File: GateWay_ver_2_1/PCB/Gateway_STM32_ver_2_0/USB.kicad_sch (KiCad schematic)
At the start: 9 parts, among them J13 USB_A, U17 TPD2EUSB30, U21 TPS2041C

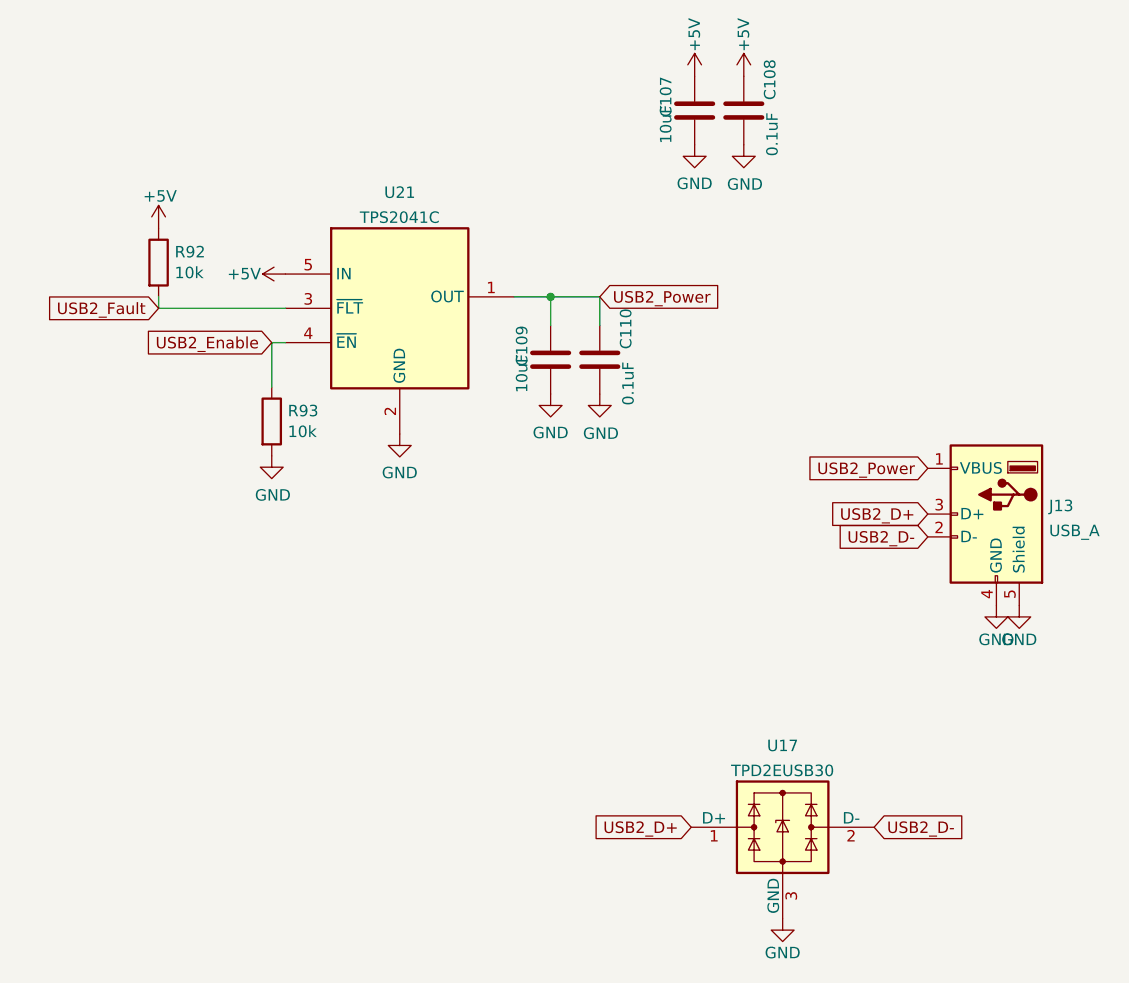
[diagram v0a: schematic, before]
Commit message: 1
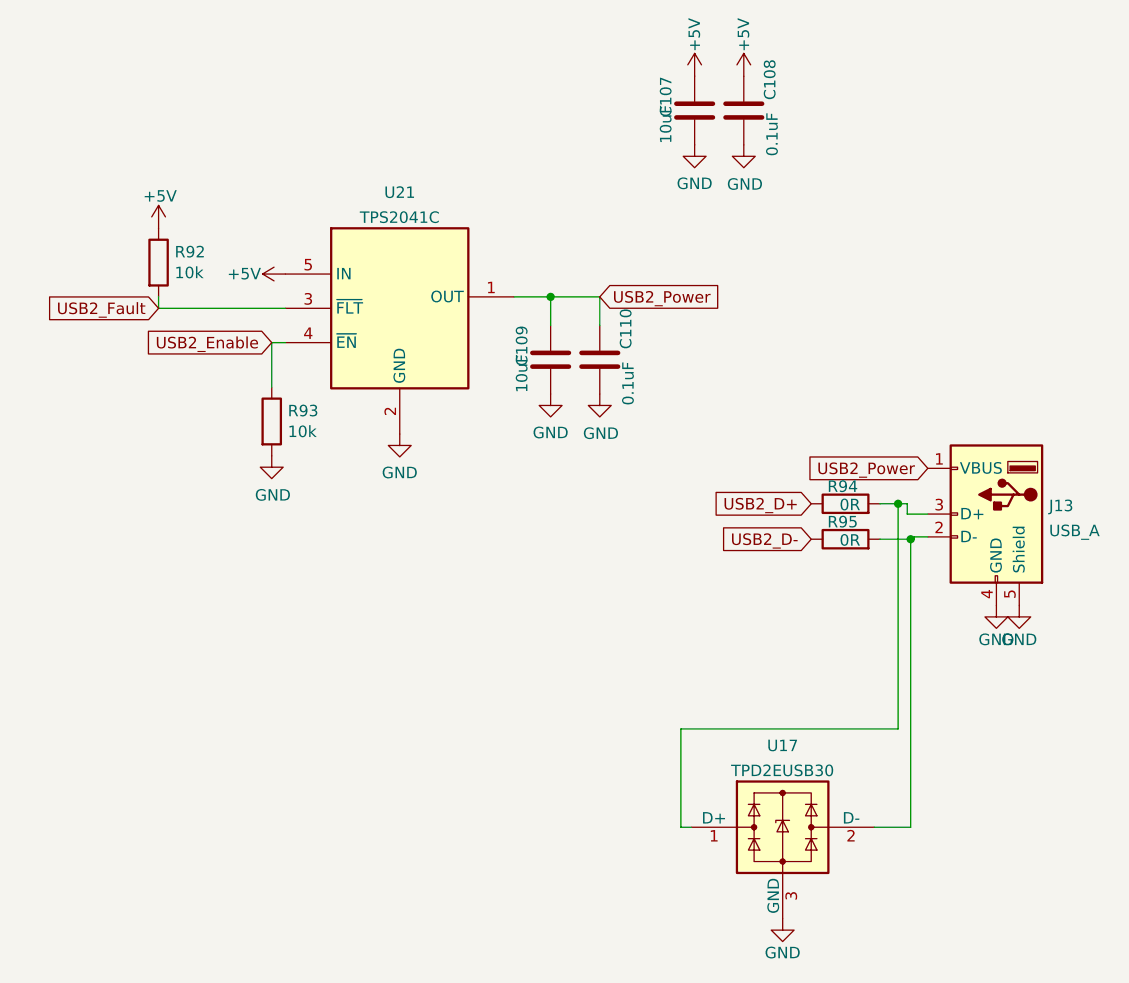
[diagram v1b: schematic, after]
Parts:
- added R94, R95: 0R, Resistor_SMD:R_0603_1608Metric, symbol Device:R
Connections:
- net USB2_D+: now also R94.1; no longer J13.3 (D+), U17.1 (D+)
- net USB2_D-: now also R95.1; no longer J13.2 (D-), U17.2 (D-)
- new net: J13.3 (D+), R94.2, U17.1 (D+)
- new net: J13.2 (D-), R95.2, U17.2 (D-)
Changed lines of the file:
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@@
 (kicad_sch (version 20211123) (generator eeschema)
   (paper "A4")
+  (junction (at 195.58 80.137) (diameter 0) (color 0 0 0 0)
+  )
   (junction (at 156.972 57.15) (diameter 0) (color 0 0 0 0)
   )
+  (junction (at 196.977 84.074) (diameter 0) (color 0 0 0 0)
+  )
+  (wire (pts (xy 195.58 105.156) (xy 195.58 80.137))
+    (stroke (width 0) (type default) (color 0 0 0 0))
+  )
+  (wire (pts (xy 171.45 105.156) (xy 195.58 105.156))
+    (stroke (width 0) (type default) (color 0 0 0 0))
+  )
   (wire (pts (xy 113.411 58.42) (xy 113.411 57.15))
     (stroke (width 0) (type default) (color 0 0 0 0))
   )
+  (wire (pts (xy 196.596 80.137) (xy 195.58 80.137))
+    (stroke (width 0) (type default) (color 0 0 0 0))
+  )
   (wire (pts (xy 125.984 62.23) (xy 125.984 67.183))
     (stroke (width 0) (type default) (color 0 0 0 0))
   )
+  (wire (pts (xy 198.882 81.28) (xy 196.596 81.28))
+    (stroke (width 0) (type default) (color 0 0 0 0))
+  )
   (wire (pts (xy 156.972 57.15) (xy 162.433 57.15))
     (stroke (width 0) (type default) (color 0 0 0 0))
   )
+  (wire (pts (xy 171.45 116.078) (xy 171.45 105.156))
+    (stroke (width 0) (type default) (color 0 0 0 0))
+  )
+  (wire (pts (xy 192.913 116.078) (xy 196.977 116.078))
+    (stroke (width 0) (type default) (color 0 0 0 0))
+  )
+  (wire (pts (xy 197.358 83.82) (xy 198.882 83.82))
+    (stroke (width 0) (type default) (color 0 0 0 0))
+  )
+  (wire (pts (xy 195.58 80.137) (xy 193.548 80.137))
+    (stroke (width 0) (type default) (color 0 0 0 0))
+  )
+  (wire (pts (xy 196.977 116.078) (xy 196.977 84.074))
+    (stroke (width 0) (type default) (color 0 0 0 0))
+  )
+  (wire (pts (xy 196.977 84.074) (xy 197.358 84.074))
+    (stroke (width 0) (type default) (color 0 0 0 0))
+  )
   (wire (pts (xy 156.972 57.15) (xy 156.972 60.325))
     (stroke (width 0) (type default) (color 0 0 0 0))
@@
     (stroke (width 0) (type default) (color 0 0 0 0))
   )
+  (wire (pts (xy 172.593 116.078) (xy 171.45 116.078))
+    (stroke (width 0) (type default) (color 0 0 0 0))
+  )
+  (wire (pts (xy 196.596 81.28) (xy 196.596 80.137))
+    (stroke (width 0) (type default) (color 0 0 0 0))
+  )
+  (wire (pts (xy 197.358 84.074) (xy 197.358 83.82))
+    (stroke (width 0) (type default) (color 0 0 0 0))
+  )
   (wire (pts (xy 127.508 58.42) (xy 113.411 58.42))
     (stroke (width 0) (type default) (color 0 0 0 0))
   )
-  (global_label "USB2_D-" (shape input) (at 192.913 116.078 0) (fields_autoplaced)
-    (effects (font (size 1.27 1.27)) (justify left))
-    (property "Intersheet References" "${INTERSHEET_REFS}" (id 0) (at 204.0667 116.1574 0)
-      (effects (font (size 1.27 1.27)) (justify left) hide)
-    )
-  )
-  (global_label "USB2_D+" (shape input) (at 172.593 116.078 180) (fields_autoplaced)
-    (effects (font (size 1.27 1.27)) (justify right))
-    (property "Intersheet References" "${INTERSHEET_REFS}" (id 0) (at 161.4393 115.9986 0)
-      (effects (font (size 1.27 1.27)) (justify right) hide)
-    )
-  )
-  (global_label "USB2_D+" (shape input) (at 198.882 81.28 180) (fields_autoplaced)
-    (effects (font (size 1.27 1.27)) (justify right))
-    (property "Intersheet References" "${INTERSHEET_REFS}" (id 0) (at 187.7283 81.2006 0)
-      (effects (font (size 1.27 1.27)) (justify right) hide)
-    )
-  )
-  (global_label "USB2_D-" (shape input) (at 198.882 83.82 180) (fields_autoplaced)
-    (effects (font (size 1.27 1.27)) (justify right))
-    (property "Intersheet References" "${INTERSHEET_REFS}" (id 0) (at 187.7283 83.7406 0)
+  (wire (pts (xy 193.548 84.074) (xy 196.977 84.074))
+    (stroke (width 0) (type default) (color 0 0 0 0))
+  )
+  (global_label "USB2_D+" (shape input) (at 185.928 80.137 180) (fields_autoplaced)
+    (effects (font (size 1.27 1.27)) (justify right))
+    (property "Intersheet References" "${INTERSHEET_REFS}" (id 0) (at 174.7743 80.0576 0)
+      (effects (font (size 1.27 1.27)) (justify right) hide)
+    )
+  )
+  (global_label "USB2_D-" (shape input) (at 185.928 84.074 180) (fields_autoplaced)
+    (effects (font (size 1.27 1.27)) (justify right))
+    (property "Intersheet References" "${INTERSHEET_REFS}" (id 0) (at 174.7743 83.9946 0)
       (effects (font (size 1.27 1.27)) (justify right) hide)
     )
@@
     )
     (property "Datasheet" "~" (id 3) (at 172.974 36.449 0)
+      (effects (font (size 1.27 1.27)) hide)
+    )
+    (pin "1")
+    (pin "2")
+  )
+  (symbol (lib_id "Device:R") (at 189.738 80.137 90) (unit 1)
+    (in_bom yes) (on_board yes)
+    (property "Reference" "R94" (id 0) (at 191.135 78.232 90)
+      (effects (font (size 1.27 1.27)) (justify left))
+    )
+    (property "Value" "0R" (id 1) (at 191.389 80.264 90)
+      (effects (font (size 1.27 1.27)) (justify left))
+    )
+    (property "Footprint" "Resistor_SMD:R_0603_1608Metric" (id 2) (at 189.738 81.915 90)
+      (effects (font (size 1.27 1.27)) hide)
+    )
+    (property "Datasheet" "~" (id 3) (at 189.738 80.137 0)
       (effects (font (size 1.27 1.27)) hide)
     )
@@
     (pin "5")
   )
+  (symbol (lib_id "Device:R") (at 189.738 84.074 90) (unit 1)
+    (in_bom yes) (on_board yes)
+    (property "Reference" "R95" (id 0) (at 191.135 82.169 90)
+      (effects (font (size 1.27 1.27)) (justify left))
+    )
+    (property "Value" "0R" (id 1) (at 191.389 84.201 90)
+      (effects (font (size 1.27 1.27)) (justify left))
+    )
+    (property "Footprint" "Resistor_SMD:R_0603_1608Metric" (id 2) (at 189.738 85.852 90)
+      (effects (font (size 1.27 1.27)) hide)
+    )
+    (property "Datasheet" "~" (id 3) (at 189.738 84.074 0)
+      (effects (font (size 1.27 1.27)) hide)
+    )
+    (pin "1")
+    (pin "2")
+  )
   (symbol (lib_id "power:GND") (at 178.435 40.259 0) (unit 1)
